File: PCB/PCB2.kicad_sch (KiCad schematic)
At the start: 8 parts, among them J1 USB_C_Receptacle_PowerOnly_6P

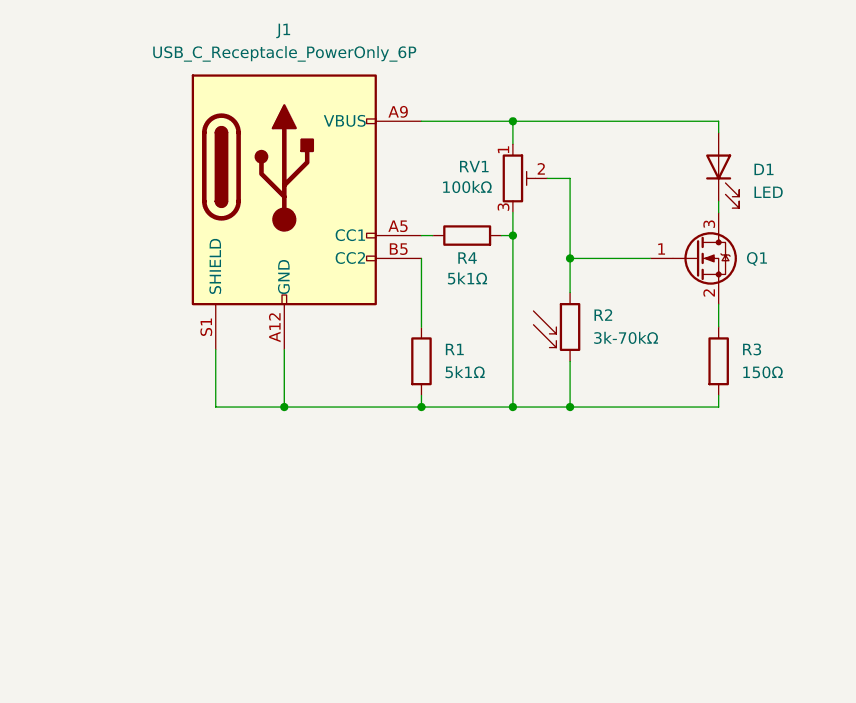
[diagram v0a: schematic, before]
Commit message: Rebuilt PCB
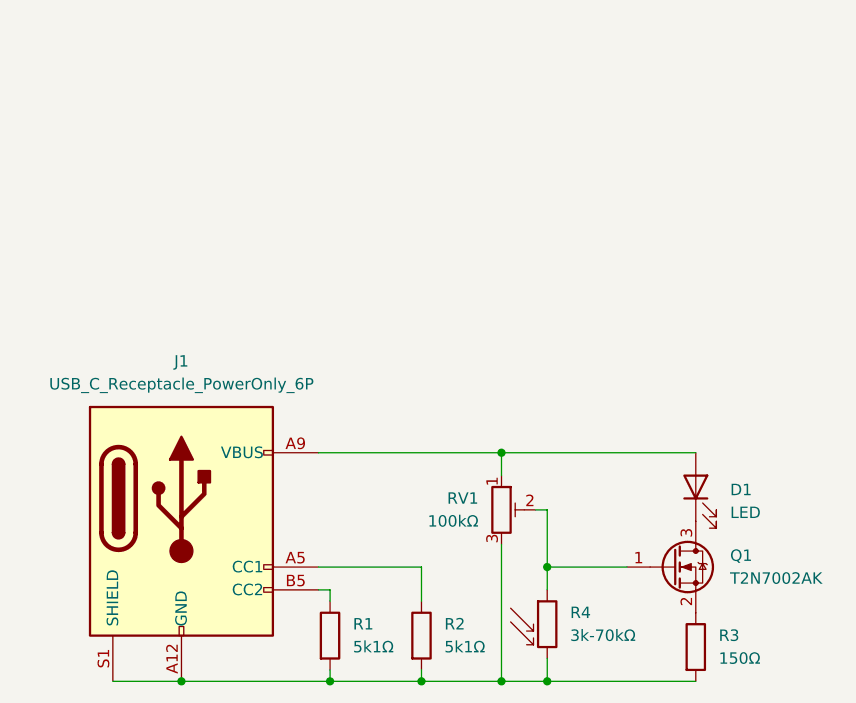
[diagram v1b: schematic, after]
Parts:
- removed R2: 3k-70kΩ, OptoDevice:R_LDR_5.1x4.3mm_P3.4mm_Vertical, symbol Sensor_Optical:LDR03
- removed R4: 5k1Ω, Resistor_SMD:R_0402_1005Metric, symbol Device:R
- added R2: 5k1Ω, Resistor_SMD:R_0402_1005Metric, symbol Device:R
- added R4: 3k-70kΩ, OptoDevice:R_LDR_5.1x4.3mm_P3.4mm_Vertical, symbol Device:R_Photo
- Q1: value ~ -> T2N7002AK
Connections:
- net at Q1.1 (G), RV1.2: now also R4.1
- net at J1.A12 (GND), J1.B12 (GND), J1.S1 (SHIELD)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: now also R2.2, R4.2
- net at J1.A5 (CC1): now also R2.1
